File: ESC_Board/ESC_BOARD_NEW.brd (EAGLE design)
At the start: 127.7 x 178 mm, 164 parts, among them J3 AVR_SPI_PROG_3X2NS, U2 ATMEGA328P_TQFP, U4 PCA9685

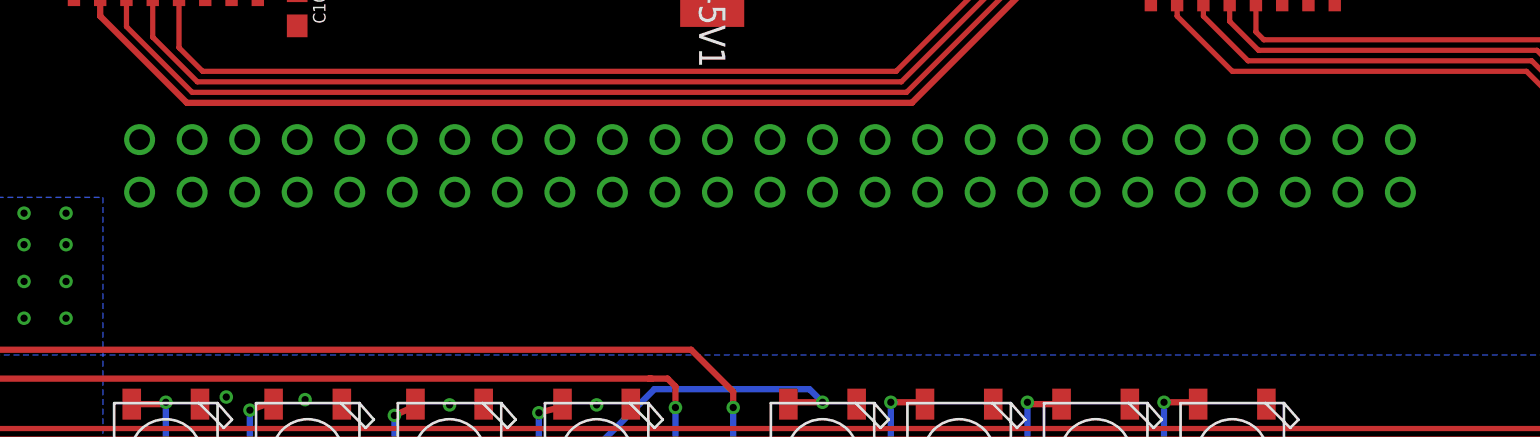
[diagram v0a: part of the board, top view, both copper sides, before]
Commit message: Some final changes
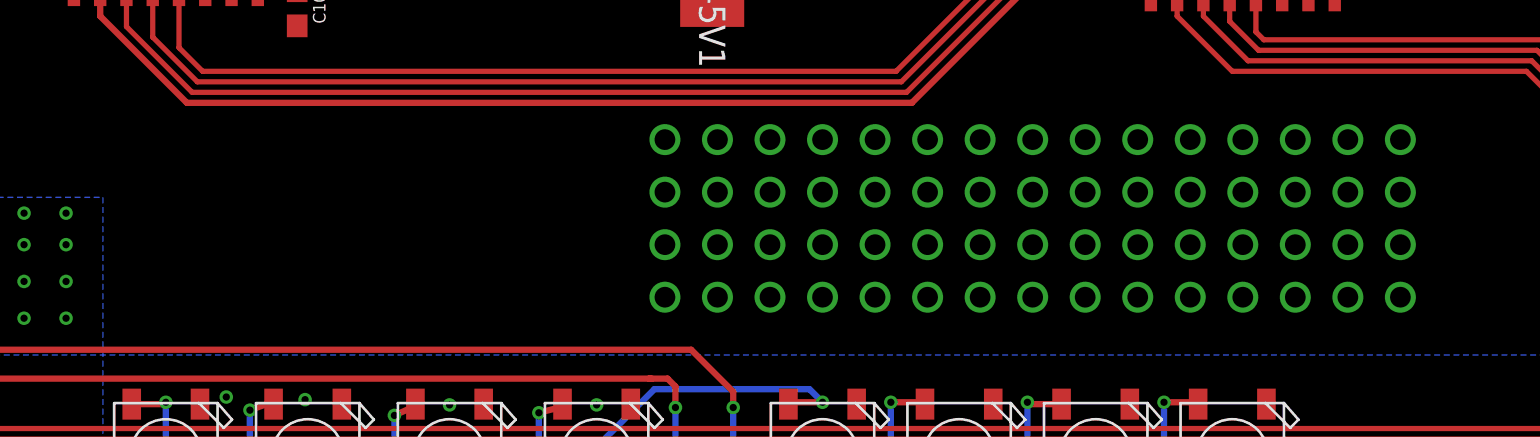
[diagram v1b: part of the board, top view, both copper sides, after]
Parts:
- U$14: value ESC-CONNECTORESC-CONNECTOR -> ESC-CONNECTORPARALLELL; device MotherboardParts:ESC-CONNECTOR -> MotherboardParts:ESC-PARALLELL
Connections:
- net +12V: now also U$14.P$101, U$14.P$102, U$14.P$103, U$14.P$104, U$14.P$105, U$14.P$106, U$14.P$107, U$14.P$108, U$14.P$109, U$14.P$110, U$14.P$111, U$14.P$112, U$14.P$113, U$14.P$114, U$14.P$115, U$14.P$116, U$14.P$117, U$14.P$118, U$14.P$119, U$14.P$120, U$14.P$121, U$14.P$122, U$14.P$123, U$14.P$124, U$14.P$125, U$14.P$126, U$14.P$127, U$14.P$128, U$14.P$129, U$14.P$130; no longer U$14.P$100, U$14.P$81, U$14.P$82, U$14.P$83, U$14.P$84, U$14.P$85, U$14.P$86, U$14.P$87, U$14.P$88, U$14.P$89, U$14.P$90, U$14.P$91, U$14.P$92, U$14.P$93, U$14.P$94, U$14.P$95, U$14.P$96, U$14.P$97, U$14.P$98, U$14.P$99
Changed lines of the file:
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@@
 <element name="LED8" library="microbuilder" package="WS2812B" value="WS2812B5050" x="85.852" y="22.352" rot="R270"/>
 <element name="C8" library="rcl" library_urn="urn:adsk.eagle:library:334" package="C0603" package3d_urn="urn:adsk.eagle:package:23616/2" value="0.1uF" x="88.138" y="18.034" rot="MR180"/>
-<element name="U$14" library="MotherboardParts" package="ESC-CONNECTOR" value="ESC-CONNECTORESC-CONNECTOR" x="55.372" y="173.736" rot="R90"/>
+<element name="U$14" library="MotherboardParts" package="ESC-PARALLELL" value="ESC-CONNECTORPARALLELL" x="55.372" y="173.736" rot="R90"/>
 </elements>
 <signals>
@@
 <contactref element="U$16" pad="P$8"/>
 <contactref element="U$16" pad="P$9"/>
-<contactref element="U$14" pad="P$85"/>
+<contactref element="U$14" pad="P$105"/>
 <contactref element="U$14" pad="P$73"/>
 <contactref element="U$14" pad="P$77"/>
@@
 <contactref element="U$14" pad="P$79"/>
 <contactref element="U$14" pad="P$66"/>
-<contactref element="U$14" pad="P$82"/>
-<contactref element="U$14" pad="P$81"/>
+<contactref element="U$14" pad="P$102"/>
+<contactref element="U$14" pad="P$101"/>
 <contactref element="U$14" pad="P$55"/>
 <contactref element="U$14" pad="P$60"/>
-<contactref element="U$14" pad="P$97"/>
-<contactref element="U$14" pad="P$87"/>
-<contactref element="U$14" pad="P$99"/>
-<contactref element="U$14" pad="P$83"/>
+<contactref element="U$14" pad="P$117"/>
+<contactref element="U$14" pad="P$107"/>
+<contactref element="U$14" pad="P$119"/>
+<contactref element="U$14" pad="P$103"/>
 <contactref element="U$14" pad="P$78"/>
-<contactref element="U$14" pad="P$94"/>
-<contactref element="U$14" pad="P$98"/>
+<contactref element="U$14" pad="P$114"/>
+<contactref element="U$14" pad="P$118"/>
 <contactref element="U$14" pad="P$75"/>
 <contactref element="U$14" pad="P$64"/>
-<contactref element="U$14" pad="P$89"/>
+<contactref element="U$14" pad="P$109"/>
 <contactref element="U$14" pad="P$56"/>
-<contactref element="U$14" pad="P$95"/>
+<contactref element="U$14" pad="P$115"/>
 <contactref element="U$14" pad="P$71"/>
 <contactref element="U$14" pad="P$68"/>
-<contactref element="U$14" pad="P$90"/>
+<contactref element="U$14" pad="P$110"/>
 <contactref element="U$14" pad="P$63"/>
-<contactref element="U$14" pad="P$84"/>
+<contactref element="U$14" pad="P$104"/>
 <contactref element="U$14" pad="P$61"/>
 <contactref element="U$14" pad="P$69"/>
-<contactref element="U$14" pad="P$92"/>
-<contactref element="U$14" pad="P$100"/>
+<contactref element="U$14" pad="P$112"/>
+<contactref element="U$14" pad="P$120"/>
 <contactref element="U$14" pad="P$54"/>
-<contactref element="U$14" pad="P$96"/>
+<contactref element="U$14" pad="P$116"/>
 <contactref element="U$14" pad="P$80"/>
 <contactref element="U$14" pad="P$67"/>
@@
 <contactref element="U$14" pad="P$70"/>
 <contactref element="U$14" pad="P$72"/>
-<contactref element="U$14" pad="P$91"/>
+<contactref element="U$14" pad="P$111"/>
 <contactref element="U$14" pad="P$52"/>
 <contactref element="U$14" pad="P$65"/>
-<contactref element="U$14" pad="P$86"/>
+<contactref element="U$14" pad="P$106"/>
 <contactref element="U$14" pad="P$51"/>
-<contactref element="U$14" pad="P$93"/>
-<contactref element="U$14" pad="P$88"/>
+<contactref element="U$14" pad="P$113"/>
+<contactref element="U$14" pad="P$108"/>
+<contactref element="U$14" pad="P$121"/>
+<contactref element="U$14" pad="P$122"/>
+<contactref element="U$14" pad="P$123"/>
+<contactref element="U$14" pad="P$124"/>
+<contactref element="U$14" pad="P$125"/>
+<contactref element="U$14" pad="P$126"/>
+<contactref element="U$14" pad="P$127"/>
+<contactref element="U$14" pad="P$128"/>
+<contactref element="U$14" pad="P$129"/>
+<contactref element="U$14" pad="P$130"/>
 </signal>
 <signal name="PWM2">
